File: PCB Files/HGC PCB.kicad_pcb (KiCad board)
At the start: 2 copper layers, 174.5 x 69.8 mm, 97 parts, among them J1 MPU6050, J10 Conn_01x07_Pin, J11 Conn_01x07_Pin, J12 Conn_01x04_Pin, J13 Conn_01x07_Pin, J14 USB_C_Receptacle_USB2.0_16P, J15 Conn_01x08_Pin, J16 Conn_01x08_Pin, J17 B2B-XH-A__LF__SN_, J18 B2B-XH-A__LF__SN_, J2 DISPLAY, J3 SDCARD, J4 Conn_01x07_Pin, J5 Conn_01x07_Pin, J6 Conn_01x07_Pin, J7 Conn_01x05_Pin, J8 Conn_01x05_Pin, J9 Conn_01x07_Pin, SW1 SW_SPDT, SW2 SW_Push, SW3 SW_Push, SW4 SW_Push, SW5 SW_Push, SW6 SW_Push, SW7 SW_Push, SW8 SW_Push, U1 STM32F407VGTx, U2 JOYSTICK, U3 AMS1117-3.3, U4 CP2102N-Axx-xQFN28, U5 MP1584EN-LF, Y1 Crystal_GND24

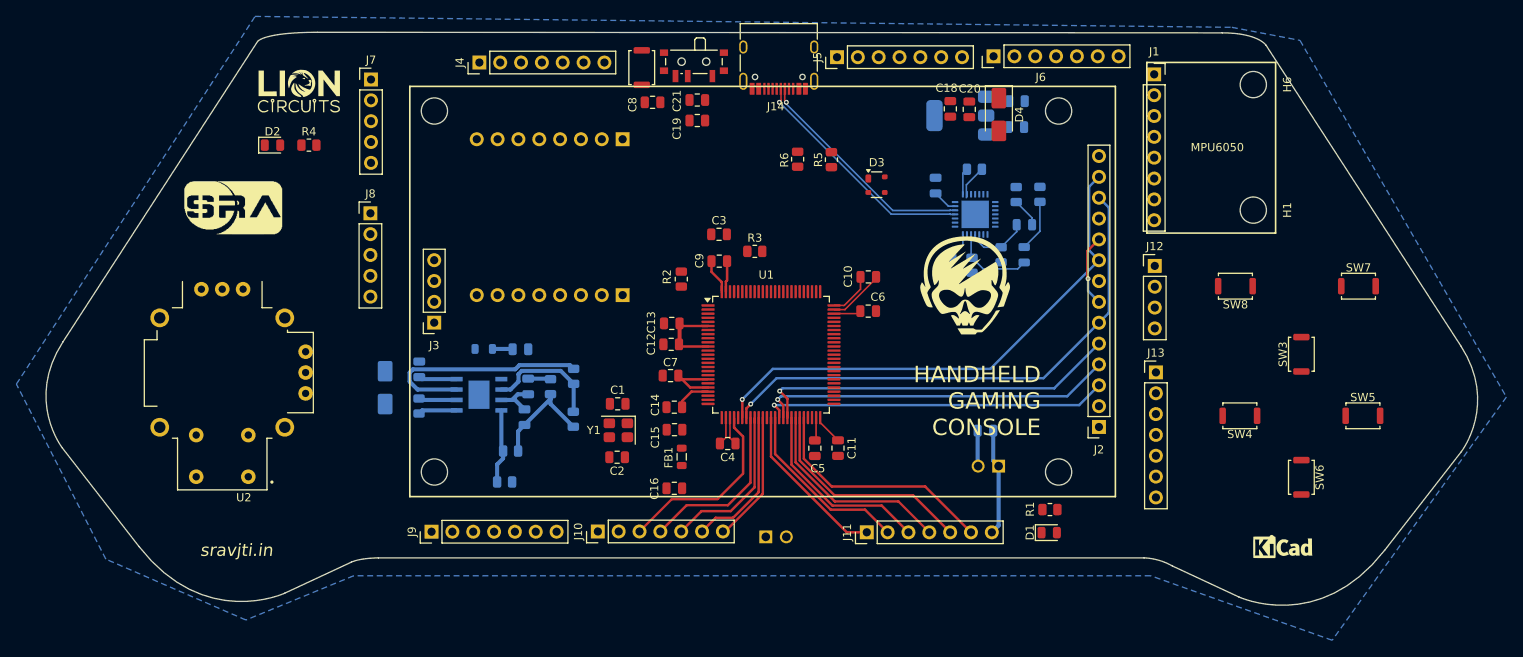
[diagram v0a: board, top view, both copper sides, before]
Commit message: Add files via upload
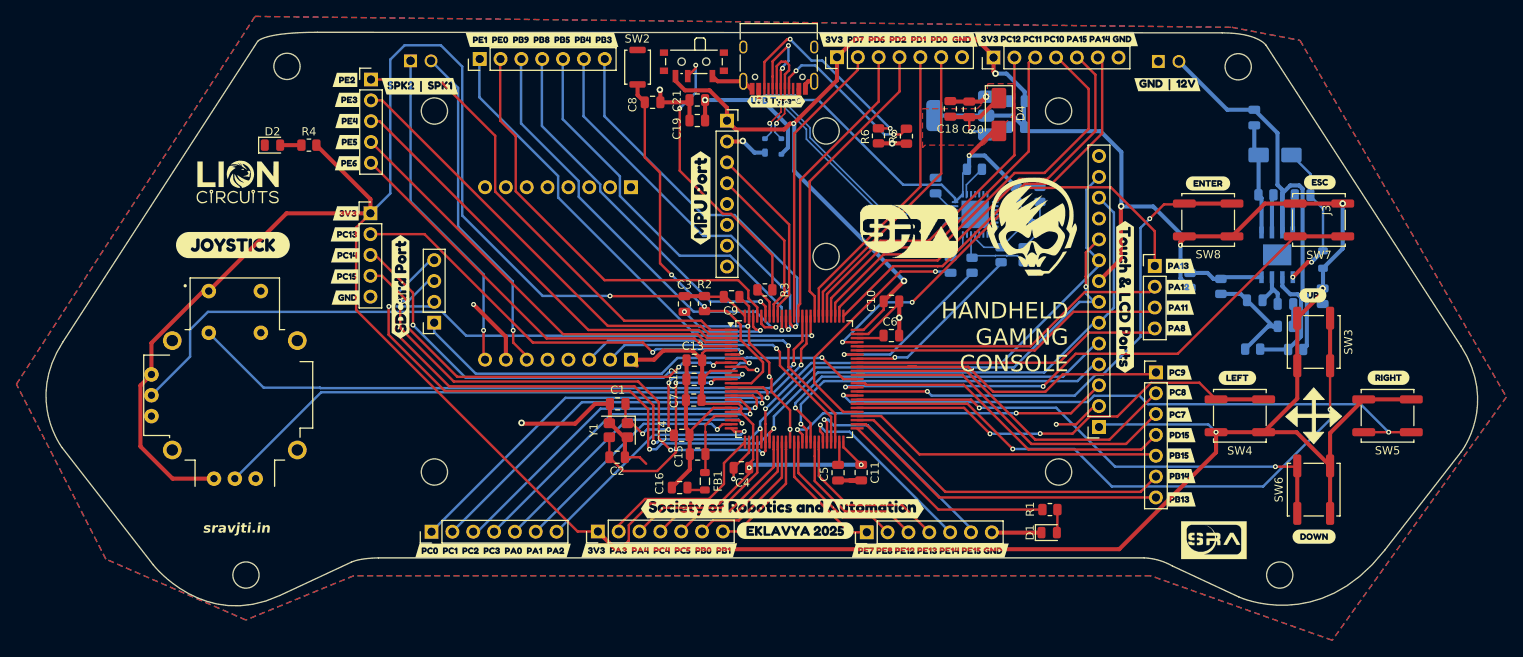
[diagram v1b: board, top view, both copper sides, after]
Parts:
- removed the G*** at (211.1, 126.5)
- added G***: LOGO, logos:sra_logo_small_neg, F.Cu at (202.7, 125.8)
- added G***: LOGO, logos:sra_skull_big, B.Cu at (154.5, 102.5)
- added G***: LOGO, Logos:sra_logo_big, B.Cu at (166.2, 109.4)
- added H10: MountingHole, MountingHole:MountingHole_3.2mm_M3, F.Cu at (107.7, 73.5)
- added H4: MountingHole, MountingHole:MountingHole_3.2mm_M3, F.Cu at (84.8, 130.0)
- added H5: MountingHole, MountingHole:MountingHole_3.2mm_M3, F.Cu at (210.8, 130.0)
- added H9: MountingHole, MountingHole:MountingHole_3.2mm_M3, F.Cu at (183.8, 73.5)
- added REF**: WEEE-Logo_8.4x12mm_SilkScreen, Symbol:WEEE-Logo_8.4x12mm_SilkScreen, B.Cu at (213.8, 121.8)
- added REF**: OSHW-Logo_7.5x8mm_SilkScreen, Symbol:OSHW-Logo_7.5x8mm_SilkScreen, B.Cu at (222.0, 119.6)
- added REF**: KiCad-Logo2_6mm_SilkScreen, symbols1:KiCad-Logo2_6mm_SilkScreen, B.Cu at (140.8, 109.5)
- added kibuzzard-668FE423: G***, kibuzzard-668FE423, F.Cu at (149.4, 72.3)
- added kibuzzard-675FDA6A: G***, kibuzzard-675FDA6A, F.Cu at (150.2, 122.0)
- added kibuzzard-68C922B8: G***, kibuzzard-68C922B8, F.Cu at (183.5, 64.7)
- added kibuzzard-68C922D4: G***, kibuzzard-68C922D4, F.Cu at (164.3, 64.8)
- added kibuzzard-68C92324: G***, kibuzzard-68C92324, F.Cu at (120.8, 64.8)
- added kibuzzard-68C923AF: G***, kibuzzard-68C923AF, F.Cu at (135.1, 127.0)
- added kibuzzard-68C923C7: G***, kibuzzard-68C923C7, F.Cu at (168.2, 127.1)
- added kibuzzard-68C923F6: G***, kibuzzard-68C923F6, F.Cu at (197.1, 70.3)
- added kibuzzard-68C92937: G***, kibuzzard-68C92937, F.Cu at (114.9, 127.1)
- added kibuzzard-68C92F98: G***, kibuzzard-68C92F98, F.Cu at (198.7, 92.3)
- added kibuzzard-68C92FA3: G***, kibuzzard-68C92FA3, F.Cu at (198.8, 94.9)
- added kibuzzard-68C92FAB: G***, kibuzzard-68C92FAB, F.Cu at (198.7, 97.4)
- added kibuzzard-68C92FB6: G***, kibuzzard-68C92FB6, F.Cu at (198.5, 99.9)
- added kibuzzard-68C92FBD: G***, kibuzzard-68C92FBD, F.Cu at (198.6, 105.3)
- added kibuzzard-68C92FC5: G***, kibuzzard-68C92FC5, F.Cu at (198.6, 107.8)
- added kibuzzard-68C92FCD: G***, kibuzzard-68C92FCD, F.Cu at (198.6, 110.5)
- added kibuzzard-68C92FD9: G***, kibuzzard-68C92FD9, F.Cu at (198.8, 113.0)
- added kibuzzard-68C92FE3: G***, kibuzzard-68C92FE3, F.Cu at (198.8, 115.5)
- added kibuzzard-68C92FEC: G***, kibuzzard-68C92FEC, F.Cu at (198.8, 118.0)
- added kibuzzard-68C92FF6: G***, kibuzzard-68C92FF6, F.Cu at (198.8, 120.8)
- added kibuzzard-68C93061: G***, kibuzzard-68C93061, F.Cu at (96.8, 69.7)
- added kibuzzard-68C93086: G***, kibuzzard-68C93086, F.Cu at (97.2, 74.7)
- added kibuzzard-68C93097: G***, kibuzzard-68C93097, F.Cu at (97.1, 72.1)
- added kibuzzard-68C930B6: G***, kibuzzard-68C930B6, F.Cu at (97.1, 79.8)
- added kibuzzard-68C930DF: G***, kibuzzard-68C930DF, F.Cu at (96.9, 86.0)
- added kibuzzard-68C930EB: G***, kibuzzard-68C930EB, F.Cu at (97.1, 77.3)
- added kibuzzard-68C93100: G***, kibuzzard-68C93100, F.Cu at (96.8, 88.5)
- added kibuzzard-68C9310A: G***, kibuzzard-68C9310A, F.Cu at (96.9, 91.1)
- added kibuzzard-68C93116: G***, kibuzzard-68C93116, F.Cu at (96.8, 93.6)
- added kibuzzard-68C93123: G***, kibuzzard-68C93123, F.Cu at (96.9, 96.2)
- added kibuzzard-68C9319C: G***, kibuzzard-68C9319C, F.Cu at (214.8, 95.9)
- added kibuzzard-68C931DF: G***, kibuzzard-68C931DF, F.Cu at (224.0, 106.0)
- added kibuzzard-68C931ED: G***, kibuzzard-68C931ED, F.Cu at (205.6, 106.0)
- added kibuzzard-68C9320A: G***, kibuzzard-68C9320A, F.Cu at (215.0, 125.3)
- added kibuzzard-68C93223: G***, kibuzzard-68C93223, F.Cu at (202.0, 82.3)
- added kibuzzard-68C9322C: G***, kibuzzard-68C9322C, F.Cu at (215.7, 82.2)
- added kibuzzard-68C9330F: G***, kibuzzard-68C9330F, F.Cu at (83.2, 89.8)
- added kibuzzard-68C93326: G***, kibuzzard-68C93326, F.Cu at (140.2, 84.1)
- added kibuzzard-68C9333E: G***, kibuzzard-68C9333E, F.Cu at (191.9, 96.1)
- added kibuzzard-68C93356: G***, kibuzzard-68C93356, F.Cu at (103.6, 94.9)
- added kibuzzard-68C938FF: G***, kibuzzard-68C938FF, B.Cu at (122.2, 78.0)
- added kibuzzard-68C939EA: G***, kibuzzard-68C939EA, F.Cu at (106.0, 70.5)
- added kibuzzard-68C93B18: G***, kibuzzard-68C93B18, B.Cu at (129.2, 106.3)
- added kibuzzard-68C93B2B: G***, kibuzzard-68C93B2B, B.Cu at (116.3, 106.3)
- added kibuzzard-68C93D93: G***, kibuzzard-68C93D93, F.Cu at (151.7, 124.6)
- D3: moved to B.Cu
- SW3, SW4, SW5, SW6, SW7, SW8: footprint Button_Switch_SMD:SW_Push_SPST_NO_Alps_SKRK -> Button_Switch_SMD:SW_Push_1P1T_NO_CK_KSC7xxJ
- moved D5 112.1 mm to (210.2, 78.8), turned to 180 degrees
- moved C22 109.7 mm to (213.6, 83.7), turned to 180 degrees
- moved R7 106.4 mm to (209.1, 83.7), turned to 0 degrees
- moved L1 102.9 mm to (216.0, 91.6), turned to -90 degrees
- moved U5 98.8 mm to (210.5, 91.0), turned to 90 degrees
- moved C29 98.0 mm to (216.0, 96.0), turned to -90 degrees
- moved C26 92.9 mm to (211.5, 97.0), turned to 0 degrees
- moved C27 90.1 mm to (207.7, 96.5), turned to 180 degrees
- moved R12 89.9 mm to (211.4, 99.7), turned to 180 degrees
- moved R11 88.9 mm to (203.6, 94.8), turned to -90 degrees
- moved R9 88.1 mm to (212.7, 102.5), turned to 180 degrees
- moved R14 87.1 mm to (199.8, 94.1), turned to -90 degrees
- moved R10 83.2 mm to (207.5, 102.5), turned to 180 degrees
- moved G*** 82.4 mm to (165.6, 88.1)
- moved J17 72.4 mm to (106.1, 66.8)
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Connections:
- SW3 pad 2: /Push1 -> /Push5
- SW4 pad 2: /Push2 -> /Push6
- SW7 pad 2: /Push5 -> /Push1
- SW8 pad 2: /Push6 -> /Push2
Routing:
- net /3.3V: track 37.2 -> 630.0 mm, vias 0 -> 11
- net GND: track 45.6 -> 179.1 mm, vias 0 -> 14
- net /SPI1_SLK: track 8.80 -> 123.7 mm, vias 1 -> 4
- net /V: track 0.00 -> 90.2 mm, vias 0 -> 1
- net /SW: track 0.00 -> 81.6 mm, vias 0 -> 1
- net /H: track 0.00 -> 81.0 mm, vias 0 -> 1
- net /Push5: track 0.00 -> 77.6 mm, vias 0 -> 2
- net /Push3: track 0.00 -> 76.5 mm, vias 0 -> 2
- net /Push1: track 0.00 -> 69.7 mm, vias 0 -> 2
- net /VBUS: track 3.26 -> 72.0 mm, vias 0 -> 4
- net /SPI1_MOSI: track 64.7 -> 130.2 mm, vias 1 -> 3
- net /Push2: track 0.00 -> 63.4 mm, vias 0 -> 2
- net /SPI1_MISO: track 63.9 -> 127.2 mm, vias 1 -> 4
- net /Push4: track 0.00 -> 62.9 mm, vias 0 -> 2
- net /PE2: track 0.00 -> 60.5 mm
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- added copper zone on F.Cu, net /5V
- added copper zone on B.Cu, net GND
- added copper zone on F.Cu, net GND
- removed copper zone on B.Cu, net (none)
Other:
- board size 174.5 x 69.8 mm -> 174.5 x 69.9 mm
- board text added: "BY, MUSTAFA T R ASHISH NERLEKAR PAARTH SHIRSAT AND MENTORS, VISHAL MUTHA PIYUSH PATLE SHAURYA RANE"
- board text added: "Designed by, Ashish N SRA VJTI Mumbai"
- board text added: "R8"
- board text removed: "By, Ashish Nerlekar Paarth Shirsat Mustafa T R"
- board text removed: "DFPLAYER-MINI"
- board text removed: "MPU6050"
